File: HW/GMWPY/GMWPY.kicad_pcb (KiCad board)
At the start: 4 copper layers, 77.4 x 77.2 mm, 87 parts, among them J1 USB_C_Receptacle, J2 Micro_SD_Card_Det, Q1 Q_PJFET_DSG, SW1 MCU_RESET, SW2 MCU_RESET, U1 AMS1117-3.3, U10 LM4040DBZ-2.0, U11 ESP32-S3-WROOM-1, U2 SRV05-4, U3 USEQGCDACH4100, U4 TSV991ILT, U5 TSV991ILT, U6 EC4-1000-H2, U7 TSV991ILT, U8 TSV991ILT, U9 TSV991ILT

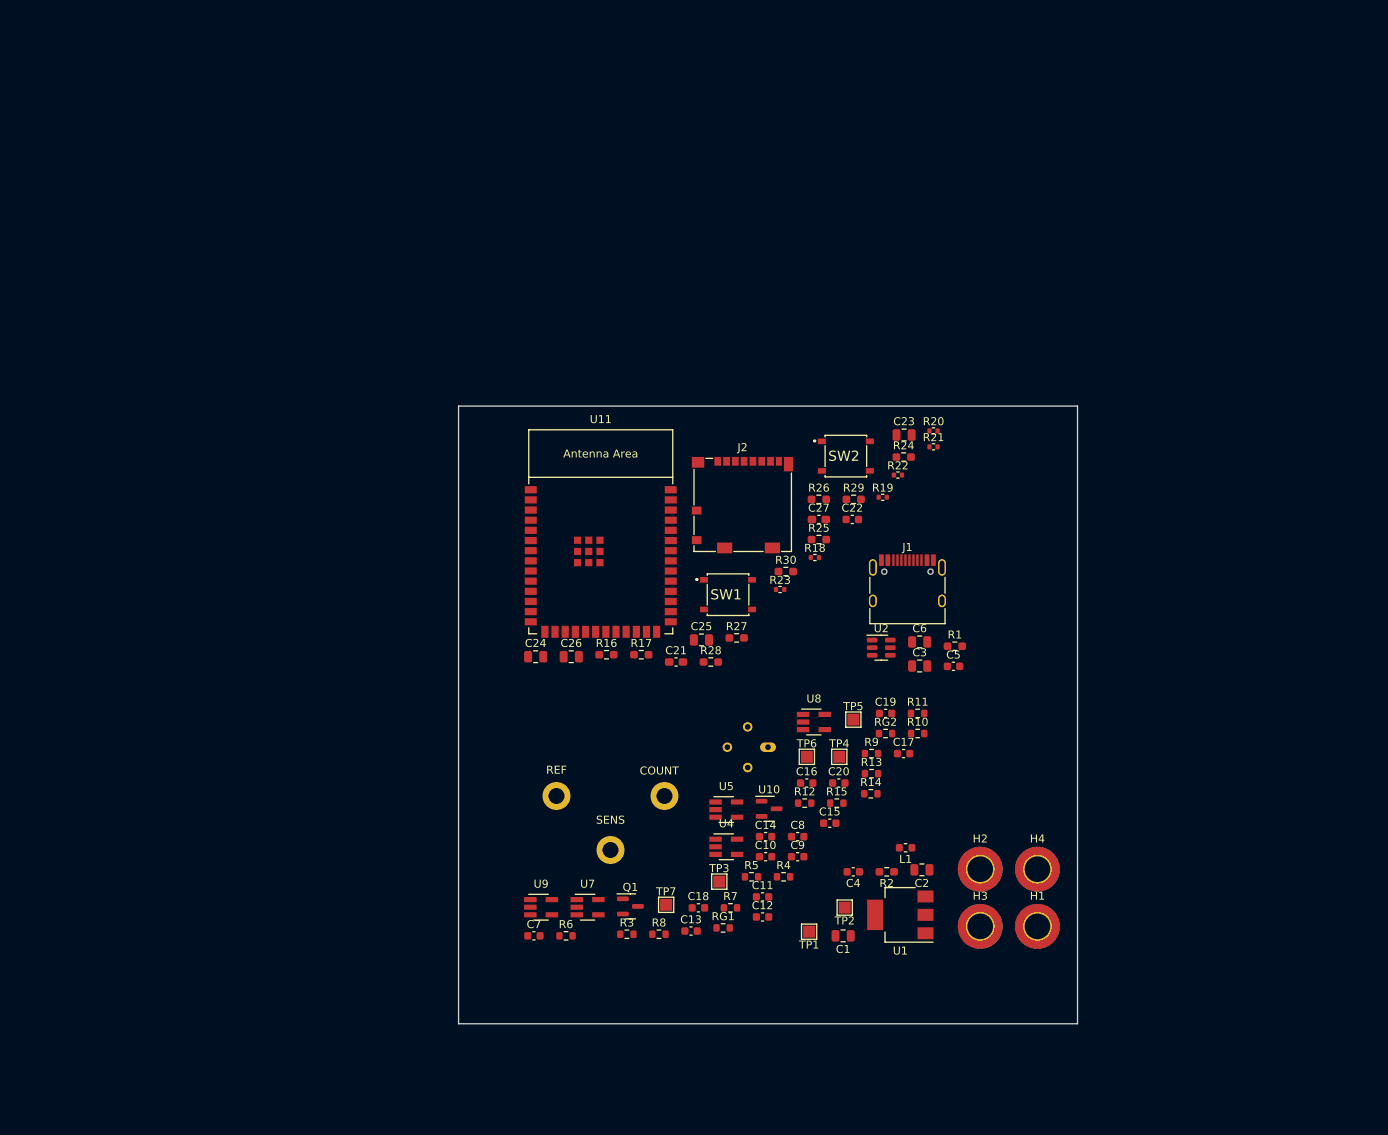
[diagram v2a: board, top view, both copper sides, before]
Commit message: b
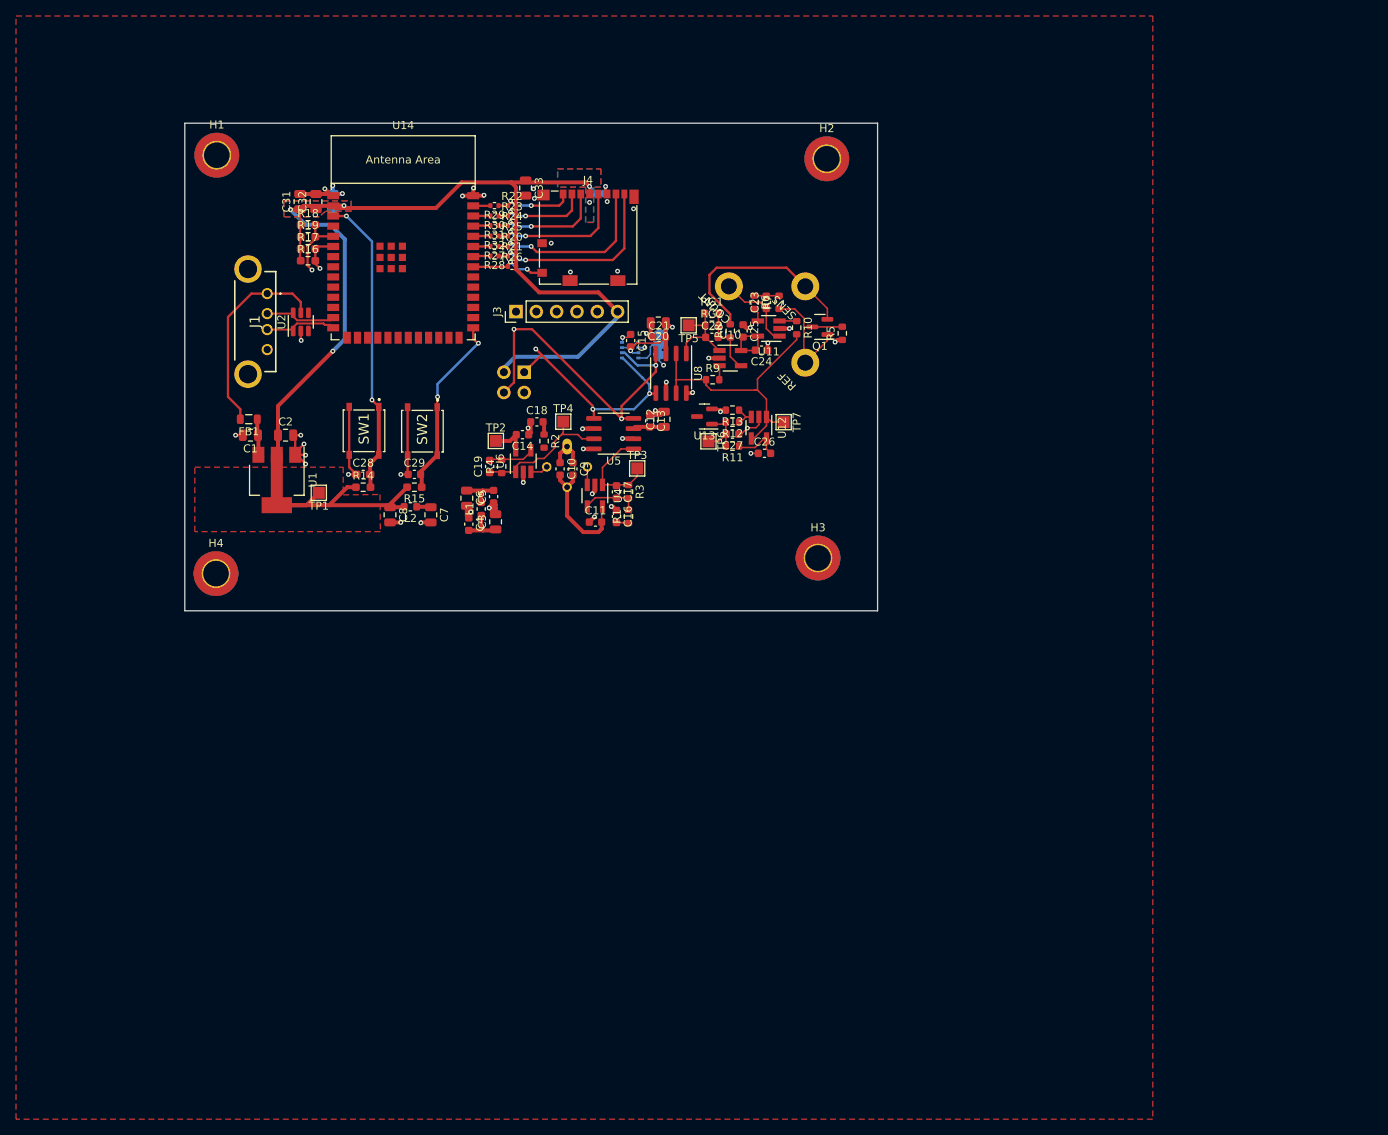
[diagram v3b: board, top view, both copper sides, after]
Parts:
- added C28: 100n, Capacitor_SMD:C_0603_1608Metric_Pad1.08x0.95mm_HandSolder, F.Cu at (72.3, 93.9)
- added C29: 2u2, Capacitor_SMD:C_0603_1608Metric, F.Cu at (78.7, 93.9)
- added C30: 10u, Capacitor_SMD:C_0805_2012Metric, B.Cu at (68.5, 59.8)
- added C31: 10u, Capacitor_SMD:C_0805_2012Metric, F.Cu at (64.4, 59.8)
- added C32: 10u, Capacitor_SMD:C_0805_2012Metric, F.Cu at (66.4, 59.8)
- added C33: 10u, Capacitor_SMD:C_0805_2012Metric, F.Cu at (92.6, 58.1)
- added C34: 100n, Capacitor_SMD:C_0603_1608Metric_Pad1.08x0.95mm_HandSolder, B.Cu at (101.7, 58.8)
- added FB1: FerriteBead_Small, Inductor_SMD:L_0805_2012Metric, F.Cu at (58.0, 87.0)
- added J3: Conn_01x10, Connector_PinHeader_2.54mm:PinHeader_1x06_P2.54mm_Vertical, F.Cu at (91.4, 73.5)
- added J4: Micro_SD_Card_Det, Connector_Card:microSD_HC_Molex_104031-0811, F.Cu at (100.4, 64.3)
- added JP1: ADR0, Jumper:SolderJumper-3_P1.3mm_Bridged12_RoundedPad1.0x1.5mm_NumberLabels, B.Cu at (109.3, 77.7)
- added L2: L_Small, Inductor_SMD:L_0603_1608Metric, F.Cu at (78.2, 98.0)
- added R31: 10, Resistor_SMD:R_0402_1005Metric, F.Cu at (88.7, 62.8)
- added R32: 10, Resistor_SMD:R_0402_1005Metric, F.Cu at (88.7, 64.1)
- added U12: TSV991ILT, Package_TO_SOT_SMD:SOT-23-5_HandSoldering, F.Cu at (121.8, 88.1)
- added U13: LM4040DBZ-2.0, Package_TO_SOT_SMD:SOT-23, F.Cu at (115.0, 86.7)
- added U14: ESP32-S3-WROOM-1, Espressif:ESP32-S3-WROOM-1, F.Cu at (77.3, 67.3)
- C12: value 3n3 -> 10u; footprint Capacitor_SMD:C_0603_1608Metric -> Capacitor_SMD:C_0805_2012Metric
- C14: value 3n3 -> 2u2
- C15, C16: value 100n -> 2u2
- C17, C19: value 2u2 -> 3n3
- C20, C7, C8: value 2u2 -> 10u; footprint Capacitor_SMD:C_0603_1608Metric -> Capacitor_SMD:C_0805_2012Metric
- C21, C27: value 100n -> 2u2; footprint Capacitor_SMD:C_0603_1608Metric_Pad1.08x0.95mm_HandSolder -> Capacitor_SMD:C_0603_1608Metric
- C22: value 2u2 -> 100n
- C23: value 10u -> 100n; footprint Capacitor_SMD:C_0805_2012Metric -> Capacitor_SMD:C_0603_1608Metric
- C24, C25, C26: value 10u -> 2u2; footprint Capacitor_SMD:C_0805_2012Metric -> Capacitor_SMD:C_0603_1608Metric
- J1: value USB_C_Receptacle -> USB_A; footprint Connector_USB:USB_C_Receptacle_HRO_TYPE-C-31-M-12 -> SamacSys_Parts:USB1040GFLB
- J2: value Micro_SD_Card_Det -> Conn_02x02_Odd_Even; footprint Connector_Card:microSD_HC_Molex_104031-0811 -> Connector_PinHeader_2.54mm:PinHeader_2x02_P2.54mm_Vertical; moved to B.Cu
- R1, R2: value 5k1 -> 56k; footprint Resistor_SMD:R_0603_1608Metric_Pad0.98x0.95mm_HandSolder -> Resistor_SMD:R_0603_1608Metric
- R10, R20, R21, R22, R23: value 10 -> 10k
- R11: value 10 -> 1k
- R12: value 10k -> 1k
- R14, R15: value 1k -> 10k; footprint Resistor_SMD:R_0603_1608Metric -> Resistor_SMD:R_0603_1608Metric_Pad0.98x0.95mm_HandSolder
- R16: value 10k -> DNP
- R18: value 10 -> 10k; footprint Resistor_SMD:R_0402_1005Metric -> Resistor_SMD:R_0603_1608Metric_Pad0.98x0.95mm_HandSolder
- R19: value 10 -> DNP; footprint Resistor_SMD:R_0402_1005Metric -> Resistor_SMD:R_0603_1608Metric_Pad0.98x0.95mm_HandSolder
- R24, R25, R26: footprint Resistor_SMD:R_0603_1608Metric_Pad0.98x0.95mm_HandSolder -> Resistor_SMD:R_0402_1005Metric
- R27, R28, R29, R30: value 10k -> 10; footprint Resistor_SMD:R_0603_1608Metric_Pad0.98x0.95mm_HandSolder -> Resistor_SMD:R_0402_1005Metric
- R3, R4: value 56k -> 1Meg
- R6, R7: value 1Meg -> 10k
- R8, R9: value 10k -> 10
- U10: value LM4040DBZ-2.0 -> TSV991ILT; footprint Package_TO_SOT_SMD:SOT-23 -> Package_TO_SOT_SMD:SOT-23-5_HandSoldering
- U11: value ESP32-S3-WROOM-1 -> TSV991ILT; footprint Espressif:ESP32-S3-WROOM-1 -> Package_TO_SOT_SMD:SOT-23-5_HandSoldering
- U5, U8: value TSV991ILT -> MCP3422; footprint Package_TO_SOT_SMD:SOT-23-5_HandSoldering -> Package_SO:SOIC-8_3.9x4.9mm_P1.27mm
- U6: value EC4-1000-H2 -> TSV991ILT; footprint Z_mycustom_footprint_lib:EC4-3pin -> Package_TO_SOT_SMD:SOT-23-5_HandSoldering; moved to F.Cu
- U7: value TSV991ILT -> BME280; footprint Package_TO_SOT_SMD:SOT-23-5_HandSoldering -> Package_LGA:Bosch_LGA-8_2.5x2.5mm_P0.65mm_ClockwisePinNumbering; moved to B.Cu
- U9: value TSV991ILT -> EC4-1000-H2; footprint Package_TO_SOT_SMD:SOT-23-5_HandSoldering -> Z_mycustom_footprint_lib:EC4-3pin; moved to B.Cu
- moved H1 140.8 mm to (54.0, 54.0)
- moved H4 109.1 mm to (53.9, 106.3)
- moved C1 97.0 mm to (58.2, 89.0)
- moved C2 96.3 mm to (62.6, 89.0), turned to 0 degrees
- moved U1 95.0 mm to (61.5, 94.6), turned to -90 degrees
- moved H2 90.8 mm to (130.2, 54.5)
- moved J1 88.3 mm to (60.3, 71.3), turned to -90 degrees
- moved U2 83.2 mm to (64.5, 74.8), turned to 90 degrees
- moved R6 82.6 mm to (121.2, 72.4), turned to -90 degrees
- moved TP1 82.3 mm to (66.8, 96.2)
- moved R19 78.9 mm to (65.4, 64.2)
- moved U9 78.1 mm to (122.8, 75.2), turned to -45 degrees
- moved RG1 76.8 mm to (115.9, 73.8)
- moved Q1 76.2 mm to (129.4, 75.5), turned to 180 degrees
- moved R8 75.9 mm to (118.2, 76.0), turned to 90 degrees
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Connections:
- C11 pad 2: Net-(C11-Pad2) -> +5V
- C12 pad 1: /GAS_Measurements/OUT2 -> +3.3VA
- C12 pad 2: /GAS_Measurements/CH4_V-ref -> GND
- C13 pad 2: Net-(C13-Pad2) -> +3.3VA
- C14 pad 1: /GAS_Measurements/OUT1 -> GND
- C14 pad 2: /GAS_Measurements/CH4_V-gas -> +5V
- C15 pad 1: /GAS_Measurements/OUT3 -> GND
- C15 pad 2: /GAS_Measurements/H2_V- -> +3.3VA
- C16 pad 1: /GAS_Measurements/H2_counter -> GND
- C17 pad 1: GND -> /GAS_Measurements/OUT2
- C17 pad 2: +5V -> /GAS_Measurements/CH4_V-ref
- C18 pad 2: +5V -> Net-(C18-Pad2)
- C19 pad 1: GND -> /GAS_Measurements/OUT1
- C19 pad 2: +5V -> /GAS_Measurements/CH4_V-gas
- C20 pad 1: GND -> +3.3VA
- C20 pad 2: 2V048 -> GND
- C21 pad 2: /MCU/ESP_EN -> +3.3VA
- C22 pad 1: GND -> /GAS_Measurements/OUT3
- C22 pad 2: /MCU/ESP_BOOT -> /GAS_Measurements/H2_V-
- C23 pad 1: +3V3 -> /GAS_Measurements/H2_counter
- C23 pad 2: GND -> Net-(C23-Pad2)
- C24 pad 1: +3V3 -> GND
- C24 pad 2: GND -> +5V
- C25 pad 1: +3V3 -> GND
- C25 pad 2: GND -> +5V
- C26 pad 1: +3V3 -> GND
- C26 pad 2: GND -> +5V
- C27 pad 1: +3V3 -> GND
- C27 pad 2: GND -> 2V048
- C7 pad 1: GND -> +3.3VA
- C7 pad 2: +5V -> GND
- C8 pad 1: GND -> +3V3
- C8 pad 2: +5V -> GND
- J2 pad 1: /MCU/DATA_2 -> GPIO_5
- J2 pad 2: /MCU/DATA_3 -> +3V3
- J2 pad 3: /MCU/CMD -> GND
- J2 pad 4: +3V3 -> GPIO_6
- R1 pad 1: /cc1 -> Net-(C16-Pad2)
- R1 pad 2: GND -> /GAS_Measurements/CH4_V-ref
- R10 pad 1: /GAS_Measurements/H2_V- -> Net-(R10-Pad1)
- R10 pad 2: /GAS_Measurements/H2_sensing -> REF
- R11 pad 1: REF -> +5V
- R11 pad 2: /GAS_Measurements/H2_V+ -> 2V048
- R12 pad 1: Net-(R12-Pad1) -> /GAS_Measurements/1V024
- R12 pad 2: REF -> 2V048
- R13 pad 1: +5V -> /GAS_Measurements/1V024
- R13 pad 2: 2V048 -> GND
- R14 pad 1: /GAS_Measurements/1V012 -> +3V3
- R14 pad 2: 2V048 -> /MCU/ESP_EN
- R15 pad 1: /GAS_Measurements/1V012 -> /MCU/ESP_BOOT
- R15 pad 2: GND -> +3V3
- R16 pad 2: /MCU/ESP_EN -> GPIO_6
- R17 pad 1: /MCU/ESP_BOOT -> +3V3
- R17 pad 2: +3V3 -> GPIO_6
- R18 pad 1: /MCU/DATA_0 -> +3V3
- R18 pad 2: GPIO_42 -> GPIO_5
- R19 pad 1: /MCU/DATA_1 -> +3V3
- R19 pad 2: GPIO_41 -> GPIO_5
- R2 pad 1: /cc2 -> Net-(C18-Pad2)
- R2 pad 2: GND -> /GAS_Measurements/CH4_V-gas
- R20 pad 1: /MCU/DATA_2 -> /MCU/DATA_0
- R20 pad 2: GPIO_1 -> +3V3
- R21 pad 1: /MCU/DATA_3 -> /MCU/DATA_1
- R21 pad 2: GPIO_2 -> +3V3
- R22 pad 1: /MCU/CMD -> /MCU/DATA_2
- R22 pad 2: GPIO_43 -> +3V3
- R23 pad 1: /MCU/CLK -> /MCU/DATA_3
- R23 pad 2: GPIO_44 -> +3V3
- R24 pad 1: /MCU/DATA_0 -> /MCU/CMD
- R25 pad 1: /MCU/DATA_1 -> /MCU/CLK
- R26 pad 1: /MCU/DATA_2 -> GPIO_40
- R27 pad 1: /MCU/DATA_3 -> /MCU/DATA_0
- R27 pad 2: +3V3 -> GPIO_42
- R28 pad 1: /MCU/CMD -> /MCU/DATA_1
- R28 pad 2: +3V3 -> GPIO_41
- R29 pad 1: /MCU/CLK -> /MCU/DATA_2
- R29 pad 2: +3V3 -> GPIO_1
- R3 pad 1: Net-(C11-Pad2) -> /GAS_Measurements/OUT2
- R30 pad 1: GPIO_40 -> /MCU/DATA_3
- R30 pad 2: +3V3 -> GPIO_2
- R4 pad 1: Net-(C13-Pad2) -> /GAS_Measurements/OUT1
- R5 pad 1: /GAS_Measurements/OUT2 -> GND
- R5 pad 2: /GAS_Measurements/CH4_V-ref -> Net-(Q1-Pad3)
- R6 pad 1: /GAS_Measurements/OUT1 -> Net-(C23-Pad2)
- R6 pad 2: /GAS_Measurements/CH4_V-gas -> Net-(R6-Pad2)
- R7 pad 1: GND -> /GAS_Measurements/H2_reference
- R7 pad 2: Net-(Q1-Pad3) -> Net-(C23-Pad2)
- R8 pad 1: Net-(C16-Pad2) -> /GAS_Measurements/H2_V-
- R8 pad 2: Net-(R8-Pad2) -> /GAS_Measurements/H2_sensing
- R9 pad 1: /GAS_Measurements/H2_reference -> REF
- R9 pad 2: Net-(C16-Pad2) -> /GAS_Measurements/H2_V+
- U10 pad 1: 2V048 -> /GAS_Measurements/OUT3
- U10 pad 3: (no net) -> /GAS_Measurements/H2_V+
- U11 pad 1: GND -> /GAS_Measurements/H2_counter
- U11 pad 2: +3V3 -> GND
- U11 pad 3: /MCU/ESP_EN -> Net-(R10-Pad1)
- U11 pad 4: GPIO_4 -> Net-(R6-Pad2)
- U11 pad 5: GPIO_5 -> +5V
- U2 pad 1: unconnected-(U2-Pad1) -> D+
- U2 pad 4: D+ -> unconnected-(U2-Pad4)
- U5 pad 1: /GAS_Measurements/OUT1 -> /GAS_Measurements/OUT2
- U5 pad 3: /GAS_Measurements/CH4_Gas -> +3.3VA
- U5 pad 4: /GAS_Measurements/CH4_V-gas -> GPIO_6
- U5 pad 5: +5V -> GPIO_5
- U6 pad 1: /GAS_Measurements/H2_reference -> /GAS_Measurements/OUT1
- U6 pad 2: /GAS_Measurements/H2_sensing -> GND
- U6 pad 3: /GAS_Measurements/H2_counter -> /GAS_Measurements/CH4_Gas
- U7 pad 1: /GAS_Measurements/OUT3 -> GND
- U7 pad 2: GND -> +3.3VA
- U7 pad 3: /GAS_Measurements/H2_V+ -> GPIO_6
- U7 pad 4: /GAS_Measurements/H2_V- -> GPIO_5
- U7 pad 5: +5V -> /GAS_Measurements/ADRESS_BME280
- U8 pad 1: /GAS_Measurements/H2_counter -> /GAS_Measurements/OUT3
- U8 pad 2: GND -> REF
- U8 pad 3: Net-(R12-Pad1) -> +3.3VA
- U8 pad 4: Net-(R8-Pad2) -> GPIO_6
- U8 pad 5: +5V -> GPIO_5
- U9 pad 1: REF -> /GAS_Measurements/H2_reference
- U9 pad 2: GND -> /GAS_Measurements/H2_sensing
- U9 pad 3: /GAS_Measurements/1V012 -> /GAS_Measurements/H2_counter
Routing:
- net +3V3: track 0.00 -> 169.0 mm, vias 0 -> 5
- net GND: track 0.00 -> 95.9 mm, vias 0 -> 49
- net GPIO_6: track 0.00 -> 81.5 mm, vias 0 -> 4
- net GPIO_5: track 0.00 -> 77.1 mm, vias 0 -> 4
- net +5V: track 0.00 -> 38.6 mm
- net /MCU/ESP_EN: track 0.00 -> 37.7 mm, vias 0 -> 2
- net REF: track 0.00 -> 35.0 mm
- net /GAS_Measurements/H2_sensing: track 0.00 -> 25.8 mm
- net VBUS: track 0.00 -> 25.5 mm
- net /MCU/DATA_1: track 0.00 -> 23.8 mm, vias 0 -> 2
- net /MCU/ESP_BOOT: track 0.00 -> 23.3 mm, vias 0 -> 2
- net +3.3VA: track 0.00 -> 21.8 mm, vias 0 -> 2
- net /MCU/DATA_0: track 0.00 -> 21.8 mm, vias 0 -> 2
- net /GAS_Measurements/OUT1: track 0.00 -> 17.8 mm
- net /MCU/CLK: track 0.00 -> 17.7 mm, vias 0 -> 2
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- added copper zone on B.Cu, net +3V3
- added copper zone on F.Cu, net +3V3
- added copper zone on F.Cu, net GND
- added copper zone on In1.Cu, net GND
- added copper zone on In2.Cu, net GND
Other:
- board size 77.4 x 77.2 mm -> 86.6 x 61 mm
